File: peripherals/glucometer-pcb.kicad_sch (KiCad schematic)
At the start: 22 parts, among them IC1 RC4558IP, IC2 LM1458N, IC3 RC4558IP, U1 ESP32_DevKit_V1_DOIT

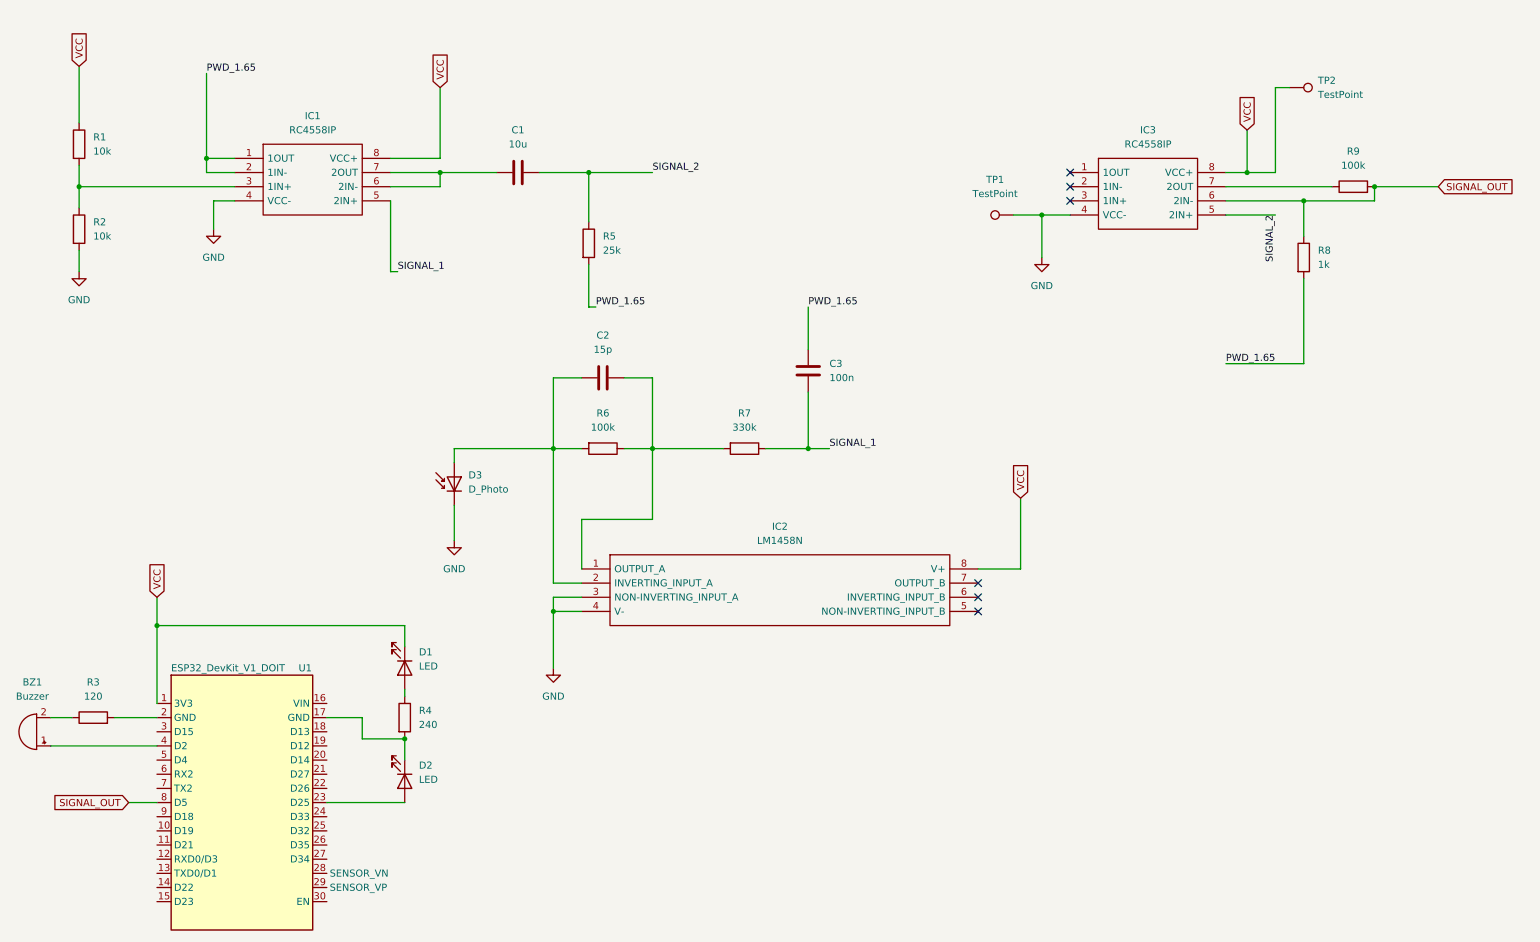
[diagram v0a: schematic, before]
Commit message: emmiter circuit
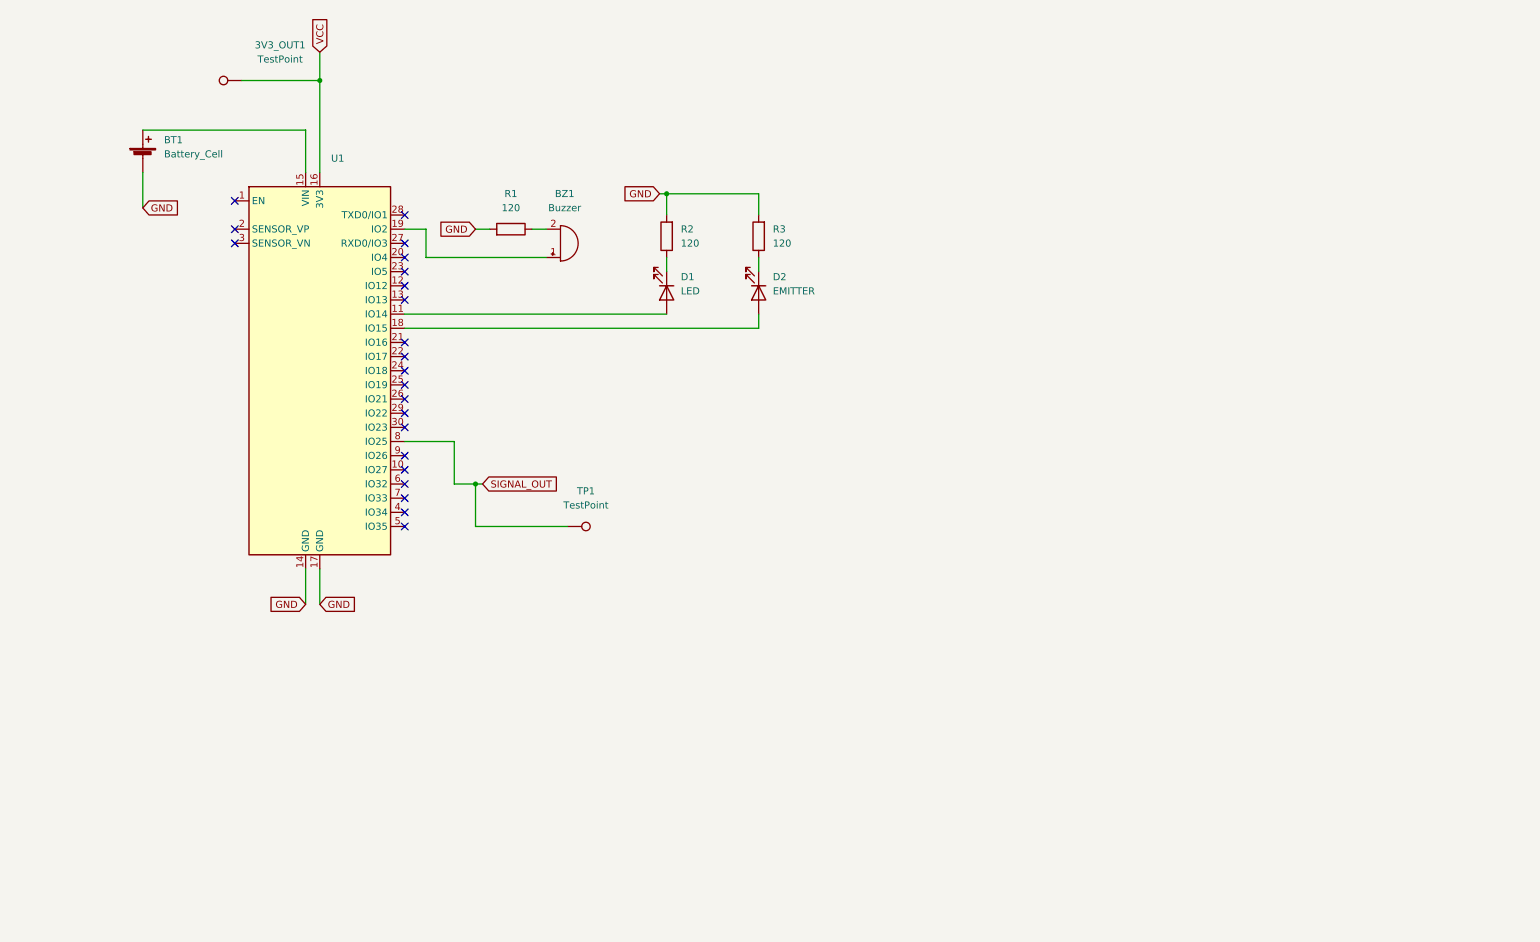
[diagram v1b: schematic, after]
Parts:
- removed C1: 10u, Capacitor_THT:CP_Radial_Tantal_D7.0mm_P5.00mm, symbol Device:C
- removed C2: 15p, Capacitor_THT:CP_Radial_D8.0mm_P3.80mm, symbol Device:C
- removed C3: 100n, Capacitor_THT:CP_Radial_Tantal_D7.0mm_P5.00mm, symbol Device:C
- removed D3: D_Photo, LED_SMD:LED_2010_5025Metric, symbol Device:D_Photo
- removed IC1, IC3: RC4558IP, Custom:DIP794W53P254L959H508Q8N, symbol RC4558IP:RC4558IP
- removed IC2: LM1458N, Custom:MC1458N, symbol LM1458N:LM1458N
- removed R1, R2: 10k, Resistor_THT:R_Axial_DIN0204_L3.6mm_D1.6mm_P7.62mm_Horizontal, symbol Device:R
- removed R5: 25k, Resistor_THT:R_Axial_DIN0204_L3.6mm_D1.6mm_P7.62mm_Horizontal, symbol Device:R
- removed R6, R9: 100k, Resistor_THT:R_Axial_DIN0204_L3.6mm_D1.6mm_P7.62mm_Horizontal, symbol Device:R
- removed R7: 330k, Resistor_THT:R_Axial_DIN0204_L3.6mm_D1.6mm_P7.62mm_Horizontal, symbol Device:R
- removed R8: 1k, Resistor_THT:R_Axial_DIN0204_L3.6mm_D1.6mm_P7.62mm_Horizontal, symbol Device:R
- removed TP2: TestPoint, TestPoint:TestPoint_Keystone_5015_Micro-Minature, symbol Connector:TestPoint
- added 3V3_OUT1: TestPoint, TestPoint:TestPoint_Keystone_5015_Micro-Minature, symbol Connector:TestPoint
- added BT1: Battery_Cell, Connector_Wire:SolderWire-0.1sqmm_1x02_P3.6mm_D0.4mm_OD1mm, symbol Device:Battery_Cell
- added R3: 120, Resistor_THT:R_Axial_DIN0204_L3.6mm_D1.6mm_P7.62mm_Horizontal, symbol Device:R
- D2: renamed from D1; value LED -> EMITTER
- R2: renamed from R4; value 240 -> 120
- U1: value ESP32_DevKit_V1_DOIT -> (none); footprint esp32_devkit_v1_doit:esp32_devkit_v1_doit -> (none)
- renumbered D2 to D1, R3 to R1
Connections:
- net GND: now also R1.2, R2.2, U1.14 (GND), U1.17 (GND), BT1.2 (-), R3.2; no longer TP1.1
- net SIGNAL_OUT: now also TP1.1
- net VCC: now also U1.16 (3V3), 3V3_OUT1.1; no longer D2.1 (K), U1.1 (3V3)
- net at D1.2 (A): now also U1.11 (IO14); no longer U1.23 (D25)
- net at U1.2 (SENSOR_VP): no longer R1.2
- net at R2.1: now also D1.1 (K); no longer D2.2 (A)
- net at BZ1.1 (-): now also U1.19 (IO2); no longer U1.4 (D2)
- net at U1.15 (VIN): now also BT1.1 (+)
- net at U1.18 (IO15): now also D2.2 (A)
- new net: D2.1 (K), R3.1
- no-connect marks 6 -> 22
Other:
- moved on the sheet: BZ1, D1, D2, R1, R2
